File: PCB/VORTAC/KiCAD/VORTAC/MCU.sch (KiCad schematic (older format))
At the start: 1 part, among them U1 STM32F103C8Tx

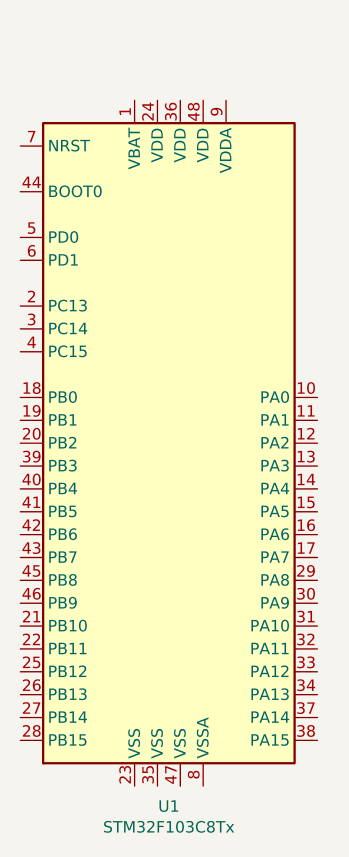
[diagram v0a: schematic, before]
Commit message: Schematic and Lib Updates
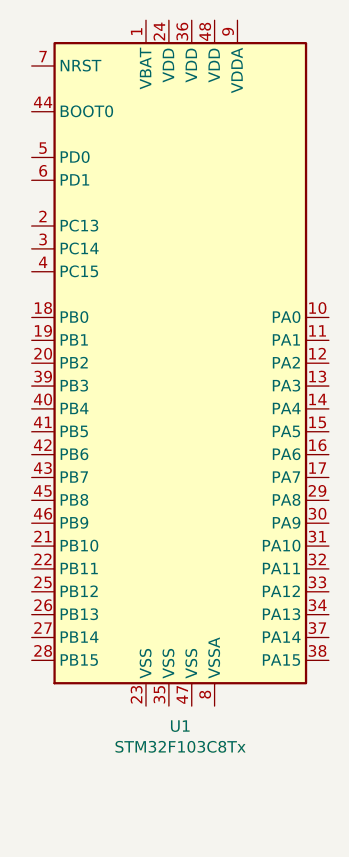
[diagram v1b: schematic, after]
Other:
- moved on the sheet: U1
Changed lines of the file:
@@
 L MCU_ST_STM32F1:STM32F103C8Tx U1
 U 1 1 6140AA25
-P 3450 3900
-F 0 "U1" H 3400 2311 50  0000 C CNN
-F 1 "STM32F103C8Tx" H 3400 2220 50  0000 C CNN
-F 2 "Package_QFP:LQFP-48_7x7mm_P0.5mm" H 2850 2500 50  0001 R CNN
-F 3 "http://www.st.com/st-web-ui/static/active/en/resource/technical/document/datasheet/CD00161566.pdf" H 3450 3900 50  0001 C CNN
-	1    3450 3900
+P 3500 3550
+F 0 "U1" H 3450 1961 50  0000 C CNN
+F 1 "STM32F103C8Tx" H 3450 1870 50  0000 C CNN
+F 2 "Package_QFP:LQFP-48_7x7mm_P0.5mm" H 2900 2150 50  0001 R CNN
+F 3 "http://www.st.com/st-web-ui/static/active/en/resource/technical/document/datasheet/CD00161566.pdf" H 3500 3550 50  0001 C CNN
+	1    3500 3550
 	1    0    0    -1
 $EndComp

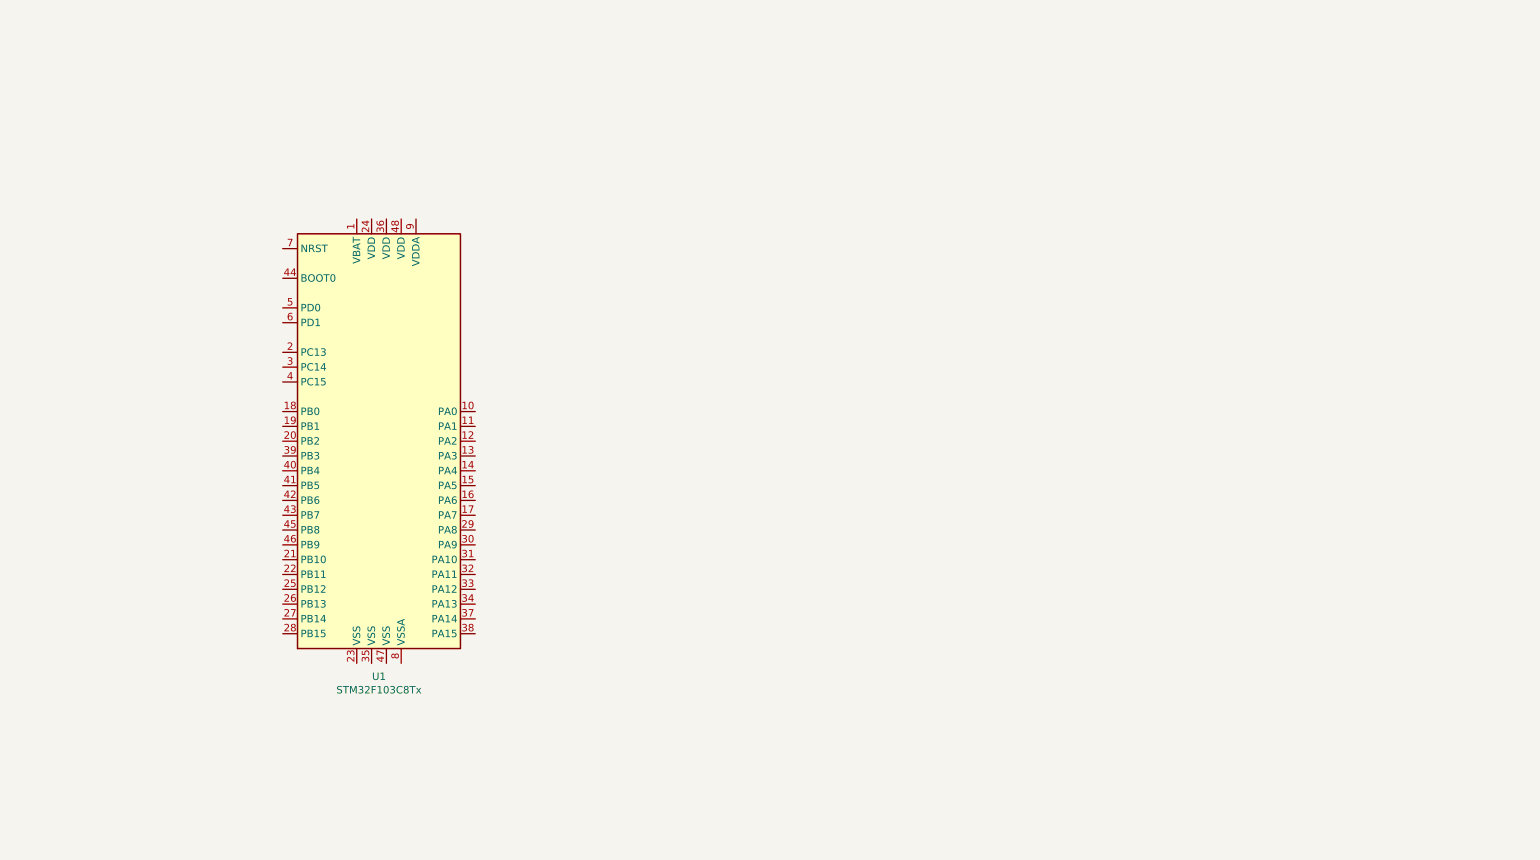
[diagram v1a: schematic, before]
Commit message: pushie
updates and stuff
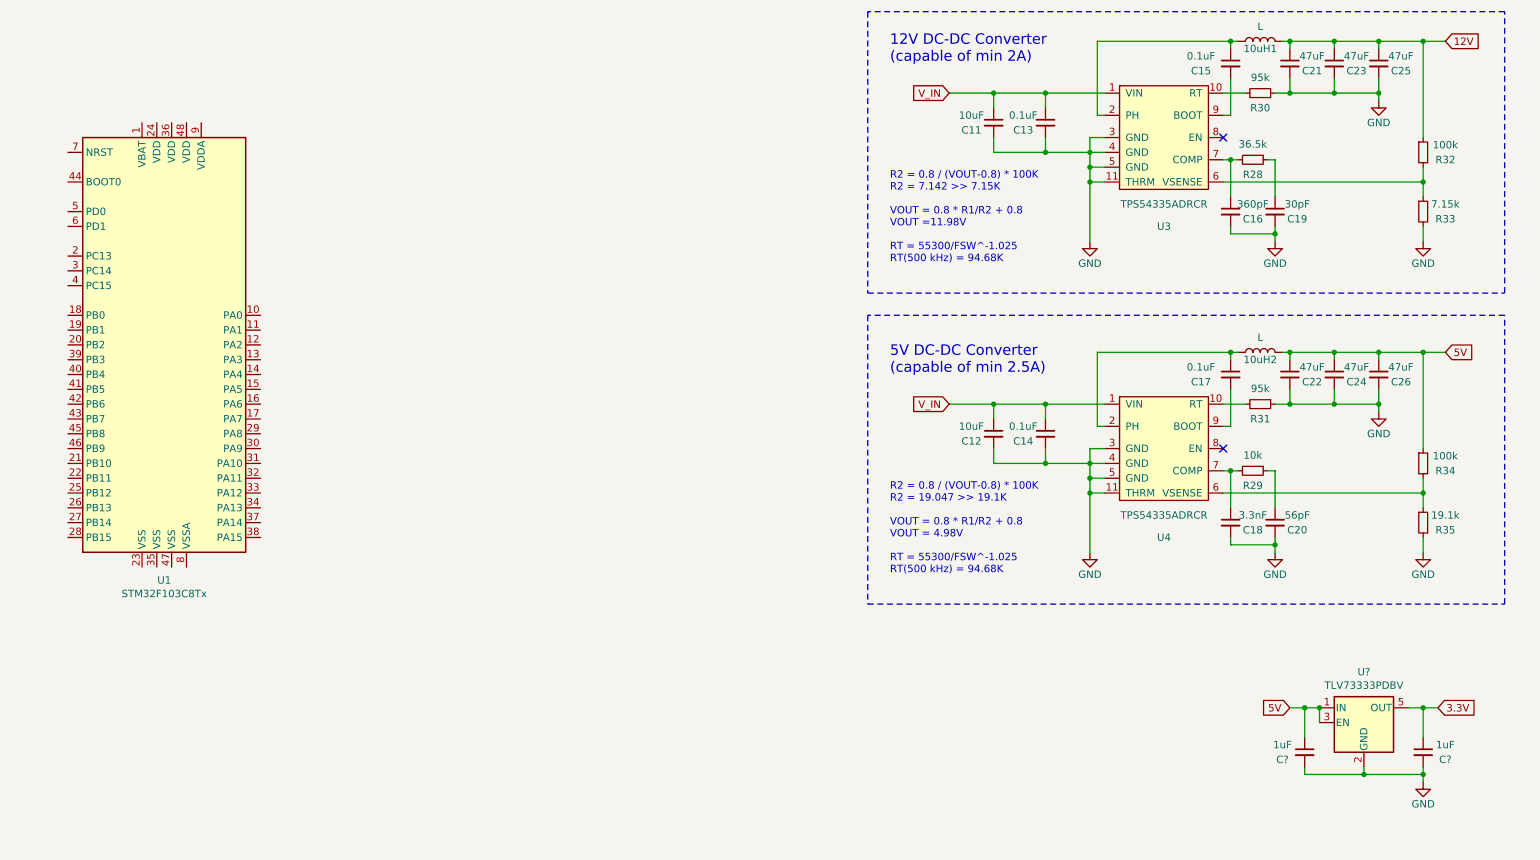
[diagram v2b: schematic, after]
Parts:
- added 10uH1, 10uH2: L, Inductor_SMD:L_Sunlord_MWSA0518_5.4x5.2mm, symbol Device:L
- added C11, C12: 10uF, Capacitor_SMD:C_1206_3216Metric, symbol Device:C_Small
- added C13, C14, C15, C17: 0.1uF, Capacitor_SMD:C_0603_1608Metric, symbol Device:C_Small
- added C16: 360pF, Capacitor_SMD:C_0603_1608Metric, symbol Device:C_Small
- added C18: 3.3nF, Capacitor_SMD:C_0603_1608Metric, symbol Device:C_Small
- added C19: 30pF, Capacitor_SMD:C_0603_1608Metric, symbol Device:C_Small
- added C20: 56pF, Capacitor_SMD:C_0603_1608Metric, symbol Device:C_Small
- added C21, C23, C25: 47uF, Capacitor_SMD:C_1206_3216Metric, symbol Device:C_Small
- added C22, C24, C26: 47uF, Capacitor_SMD:C_0805_2012Metric, symbol Device:C_Small
- added C? (x2): 1uF, Capacitor_SMD:C_0603_1608Metric, symbol Device:C_Small
- added R28: 36.5k, Resistor_SMD:R_0402_1005Metric, symbol Device:R_Small
- added R29: 10k, Resistor_SMD:R_0402_1005Metric, symbol Device:R_Small
- added R30, R31: 95k, Resistor_SMD:R_0402_1005Metric, symbol Device:R_Small
- added R32, R34: 100k, Resistor_SMD:R_0402_1005Metric, symbol Device:R_Small
- added R33: 7.15k, Resistor_SMD:R_0402_1005Metric, symbol Device:R_Small
- added R35: 19.1k, Resistor_SMD:R_0402_1005Metric, symbol Device:R_Small
- added U3, U4: TPS54335ADRCR, Package_SON:VSON-10-1EP_3x3mm_P0.5mm_EP1.65x2.4mm_ThermalVias, symbol ToolChanger:TPS54335ADRCR
- added U?: TLV73333PDBV, Package_TO_SOT_SMD:SOT-23-5, symbol Regulator_Linear:TLV73333PDBV
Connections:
- new net: R30.2, U3.10 (RT)
- new net: 10uH1.1, C15.1, U3.2 (PH)
- new net: R32.2, R33.1, U3.6 (VSENSE)
- new net: C16.1, R28.2, U3.7 (COMP)
- new net: C15.2, U3.9 (BOOT)
- new net: C19.1, R28.1
- new net: R31.2, U4.10 (RT)
- new net: 10uH2.1, C17.1, U4.2 (PH)
- new net: C17.2, U4.9 (BOOT)
- new net: C20.1, R29.1
- new net: C18.1, R29.2, U4.7 (COMP)
- new net: R34.2, R35.1, U4.6 (VSENSE)
- new net 12V: 10uH1.2, C21.1, C23.1, C25.1, R32.1
- new net 3.3V: C?.1, U?.5 (OUT)
- new net 5V: 10uH2.2, C22.1, C24.1, C26.1, C?.1, R34.1, U?.1 (IN), U?.3 (EN)
- new net GND: C11.2, C12.2, C13.2, C14.2, C16.2, C18.2, C19.2, C20.2, C21.2, C22.2, C23.2, C24.2, C25.2, C26.2, C?.2, C?.2, R30.1, R31.1, R33.2, R35.2, U3.11 (THRM), U3.3 (GND), U3.4 (GND), U3.5 (GND), U4.11 (THRM), U4.3 (GND), U4.4 (GND), U4.5 (GND), U?.2 (GND)
- new net V_IN: C11.1, C12.1, C13.1, C14.1, U3.1 (VIN), U4.1 (VIN)
- no-connect marks 0 -> 2
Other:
- note added: "12V DC-DC Converter\n(capable of min 2A)"
- note added: "5V DC-DC Converter\n(capable of min 2.5A)"
- note added: "R2 = 0.8 / (VOUT-0.8) * 100K\nR2 = 19.047 >> 19.1K\n\nVOUT = 0.8 * R1/R2 + 0.8\nVOUT = 4.98V\n\nRT = 55300/FSW^-1.025\nRT(500 kHz) = 94.68K"
- note added: "R2 = 0.8 / (VOUT-0.8) * 100K\nR2 = 7.142 >> 7.15K\n\nVOUT = 0.8 * R1/R2 + 0.8\nVOUT =11.98V\n\nRT = 55300/FSW^-1.025\nRT(500 kHz) = 94.68K"
- moved on the sheet: U1

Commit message: progress
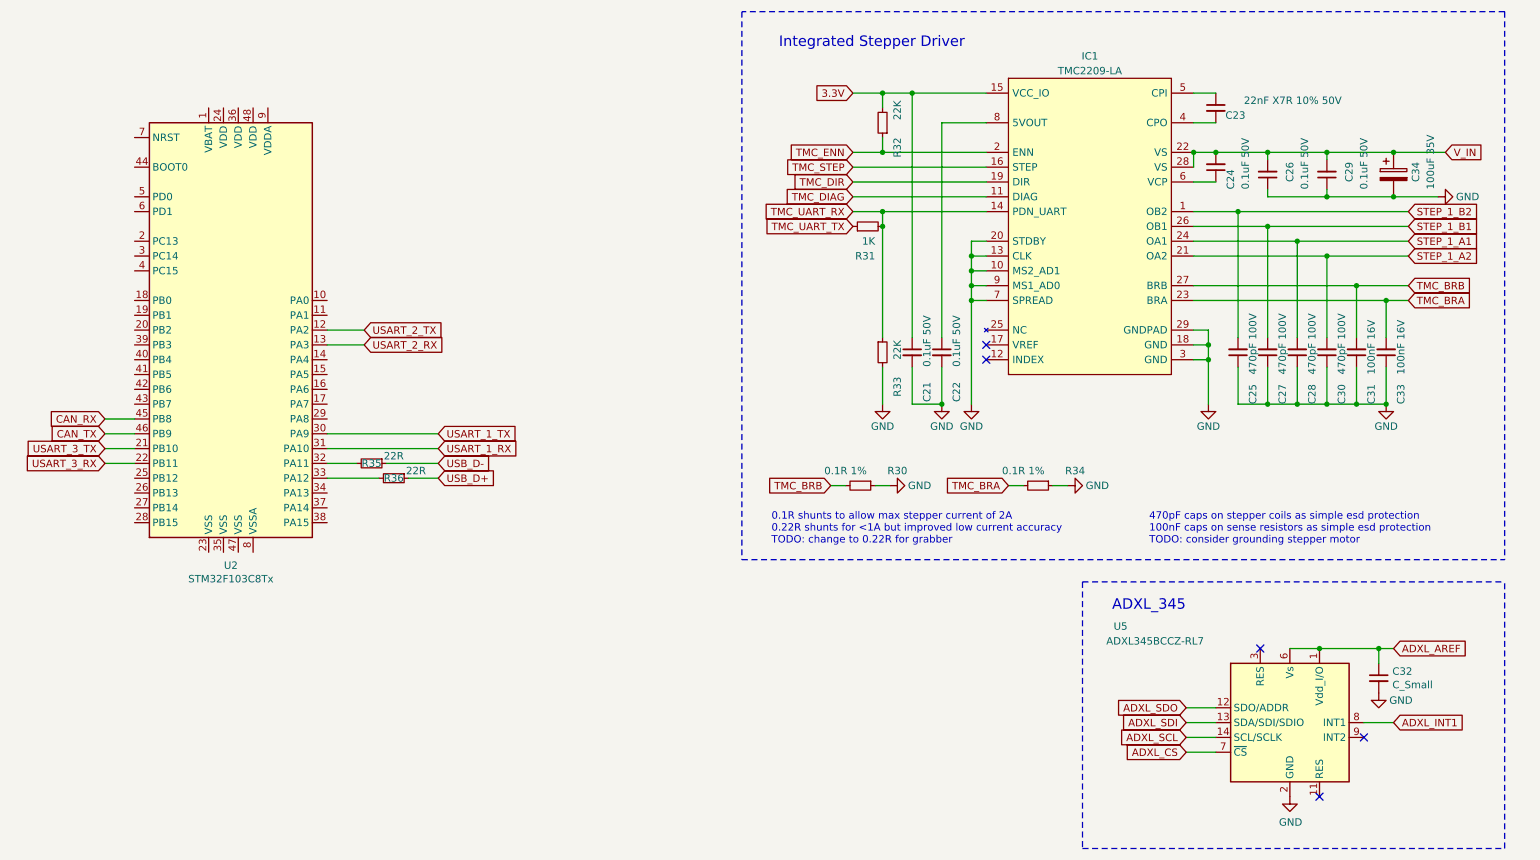
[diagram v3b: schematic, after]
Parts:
- removed 10uH1, 10uH2: L, Inductor_SMD:L_Sunlord_MWSA0518_5.4x5.2mm, symbol Device:L
- removed C11, C12: 10uF, Capacitor_SMD:C_1206_3216Metric, symbol Device:C_Small
- removed C13, C14, C15, C17: 0.1uF, Capacitor_SMD:C_0603_1608Metric, symbol Device:C_Small
- removed C16: 360pF, Capacitor_SMD:C_0603_1608Metric, symbol Device:C_Small
- removed C18: 3.3nF, Capacitor_SMD:C_0603_1608Metric, symbol Device:C_Small
- removed C19: 30pF, Capacitor_SMD:C_0603_1608Metric, symbol Device:C_Small
- removed C20: 56pF, Capacitor_SMD:C_0603_1608Metric, symbol Device:C_Small
- removed C? (x2): 1uF, Capacitor_SMD:C_0603_1608Metric, symbol Device:C_Small
- removed R28: 36.5k, Resistor_SMD:R_0402_1005Metric, symbol Device:R_Small
- removed R29: 10k, Resistor_SMD:R_0402_1005Metric, symbol Device:R_Small
- removed U3, U4: TPS54335ADRCR, Package_SON:VSON-10-1EP_3x3mm_P0.5mm_EP1.65x2.4mm_ThermalVias, symbol ToolChanger:TPS54335ADRCR
- removed U?: TLV73333PDBV, Package_TO_SOT_SMD:SOT-23-5, symbol Regulator_Linear:TLV73333PDBV
- added C27, C28, C30: 470pF 100V, Capacitor_SMD:C_0603_1608Metric, symbol Device:C_Small
- added C29: 0.1uF 50V, Capacitor_SMD:C_0603_1608Metric, symbol Device:C_Small
- added C31, C33: 100nF 16V, Capacitor_SMD:C_0603_1608Metric, symbol Device:C_Small
- added C32: C_Small, symbol Device:C_Small
- added C34: 100uF 35V, Capacitor_SMD:CP_Elec_8x6.9, symbol Device:CP
- added IC1: TMC2209-LA, ToolChanger:tmc_2209_package, symbol ToolChanger:TMC2209-LA
- added R36: 22R, Resistor_SMD:R_0402_1005Metric, symbol Device:R_Small
- added U5: ADXL345BCCZ-RL7, Package_LGA:LGA-14_3x5mm_P0.8mm_LayoutBorder1x6y, symbol Sensor_Motion:ADXL343
- C21: value 47uF -> 0.1uF 50V; footprint Capacitor_SMD:C_1206_3216Metric -> Capacitor_SMD:C_0603_1608Metric; LCSC C403725 -> (none)
- C22, C24, C26: value 47uF -> 0.1uF 50V; footprint Capacitor_SMD:C_0805_2012Metric -> Capacitor_SMD:C_0603_1608Metric; LCSC C466799 -> (none)
- C23: value 47uF -> 22nF X7R 10% 50V; footprint Capacitor_SMD:C_1206_3216Metric -> Capacitor_SMD:C_0603_1608Metric; LCSC C403725 -> (none)
- C25: value 47uF -> 470pF 100V; footprint Capacitor_SMD:C_1206_3216Metric -> Capacitor_SMD:C_0603_1608Metric; LCSC C403725 -> C437459
- R30: value 95k -> 0.1R 1%; footprint Resistor_SMD:R_0402_1005Metric -> Resistor_SMD:R_1206_3216Metric; LCSC (none) -> C346768
- R31: value 95k -> 1K; footprint Resistor_SMD:R_0402_1005Metric -> (none)
- R32: value 100k -> 22K
- R33: value 7.15k -> 22K
- R34: value 100k -> 0.1R 1%; footprint Resistor_SMD:R_0402_1005Metric -> Resistor_SMD:R_1206_3216Metric; LCSC (none) -> C346768
- R35: value 19.1k -> 22R
- renumbered U1 to U2
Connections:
- net 3.3V: now also C21.1, R32.2, IC1.15 (VCC_IO)
- net GND: now also C25.1, C26.1, R34.1, C27.1, C28.1, C29.1, C30.1, C31.1, C32.2, C33.1, C34.2, IC1.10 (MS2_AD1), IC1.13 (CLK), IC1.18 (GND), IC1.20 (STDBY), IC1.29 (GNDPAD), IC1.3 (GND), IC1.7 (SPREAD), IC1.9 (MS1_AD0), U5.2 (GND), U5.4 (GND), U5.5 (GND); no longer C23.2, C24.2, C25.2, C26.2, R31.1, R35.2
- net V_IN: now also C24.2, C26.2, C29.2, C34.1, IC1.22 (VS), IC1.28 (VS)
- net USART_2_TX: now reaches U2.12 (PA2)
- net USART_2_RX: now reaches U2.13 (PA3)
- net USART_3_TX: now reaches U2.21 (PB10)
- net USART_3_RX: now reaches U2.22 (PB11)
- net USART_1_TX: now reaches U2.30 (PA9)
- net USART_1_RX: now reaches U2.31 (PA10)
- net at U2.32 (PA11): now also R35.2
- net at U2.33 (PA12): now also R36.2
- net CAN_RX: now reaches U2.45 (PB8)
- net CAN_TX: now reaches U2.46 (PB9)
- net TMC_BRB: now reaches R30.2
- net TMC_BRB: now also C31.2, IC1.27 (BRB)
- net TMC_UART_RX: now reaches R33.1
- net TMC_UART_RX: now also R31.2, IC1.14 (PDN_UART); no longer R32.2
- net TMC_BRA: now reaches R34.2
- net TMC_BRA: now also C33.2, IC1.23 (BRA); no longer R35.1
- removed net 12V: C21.1, C23.1, C25.1, R32.1
- removed net 5V: C22.1, C24.1, C26.1, R34.1
- new net: C23.1, IC1.5 (CPI)
- new net: C23.2, IC1.4 (CPO)
- new net: C24.1, IC1.6 (VCP)
- new net: C22.1, IC1.8 (5VOUT)
- new net ADXL_AREF: C32.1, U5.1 (Vdd_I/O), U5.6 (Vs)
- new net ADXL_CS: U5.7 (~CS)
- new net ADXL_INT1: U5.8 (INT1)
- new net ADXL_SCL: U5.14 (SCL/SCLK)
- new net ADXL_SDI: U5.13 (SDA/SDI/SDIO)
- new net ADXL_SDO: U5.12 (SDO/ADDR)
- new net STEP_1_A1: C28.2, IC1.24 (OA1)
- new net STEP_1_A2: C30.2, IC1.21 (OA2)
- new net STEP_1_B1: C27.2, IC1.26 (OB1)
- new net STEP_1_B2: C25.2, IC1.1 (OB2)
- new net TMC_DIAG: IC1.11 (DIAG)
- new net TMC_DIR: IC1.19 (DIR)
- new net TMC_ENN: IC1.2 (ENN), R32.1
- new net TMC_STEP: IC1.16 (STEP)
- new net TMC_UART_TX: R31.1
- new net USB_D+: R36.1
- new net USB_D-: R35.1
- no-connect marks 2 -> 5
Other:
- note added: "0.1R shunts to allow max stepper current of 2A\n0.22R shunts for <1A but improved low current accuracy\nTODO: change to 0.22R for grabber"
- note added: "470pF caps on stepper coils as simple esd protection\n100nF caps on sense resistors as simple esd protection\nTODO: consider grounding stepper motor"
- note added: "ADXL_345"
- note added: "Integrated Stepper Driver"
- note removed: "12V DC-DC Converter\n(capable of min 2A)"
- note removed: "5V DC-DC Converter\n(capable of min 2.5A)"
- note removed: "R2 = 0.8 / (VOUT-0.8) * 100K\nR2 = 19.047 >> 19.1K\n\nVOUT = 0.8 * R1/R2 + 0.8\nVOUT = 4.98V\n\nRT = 55300/FSW^-1.025\nRT(500 kHz) = 94.68K"
- note removed: "R2 = 0.8 / (VOUT-0.8) * 100K\nR2 = 7.142 >> 7.15K\n\nVOUT = 0.8 * R1/R2 + 0.8\nVOUT =11.98V\n\nRT = 55300/FSW^-1.025\nRT(500 kHz) = 94.68K"
- moved on the sheet: U2
